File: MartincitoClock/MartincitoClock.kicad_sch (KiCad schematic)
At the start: 31 parts, among them J2 PJ-102AH, SW1 Omron_B3F_SPST, U1 ATmega328-PU, U2 L7805, Y1 Crystal

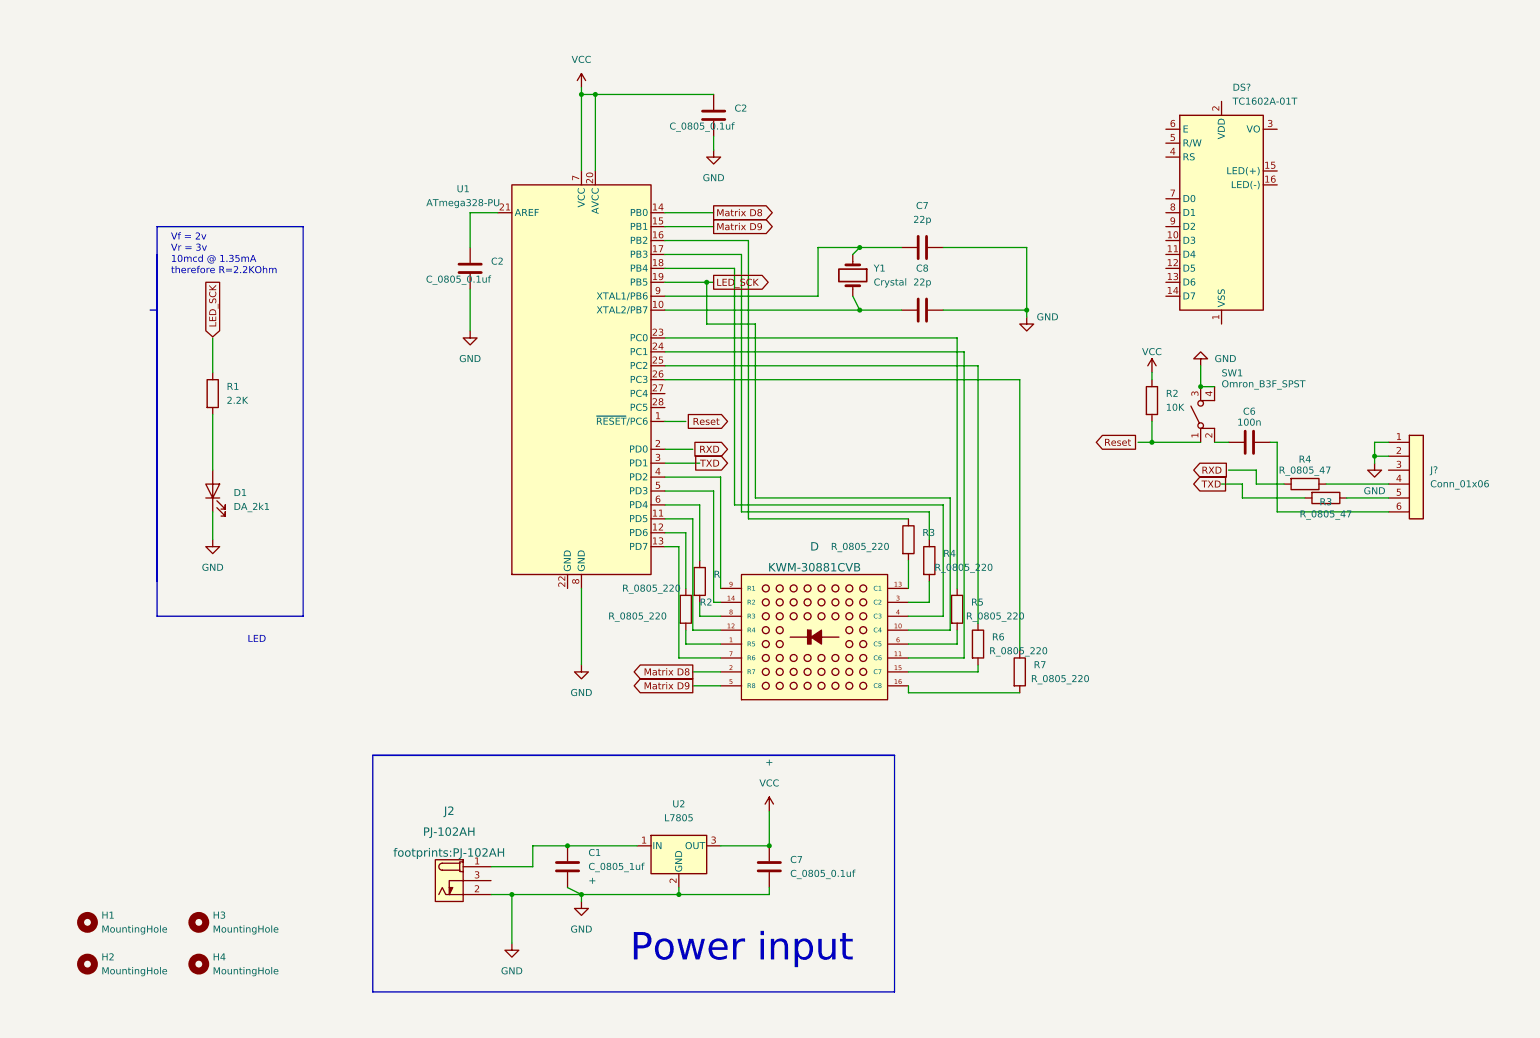
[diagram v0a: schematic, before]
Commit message: Week 5
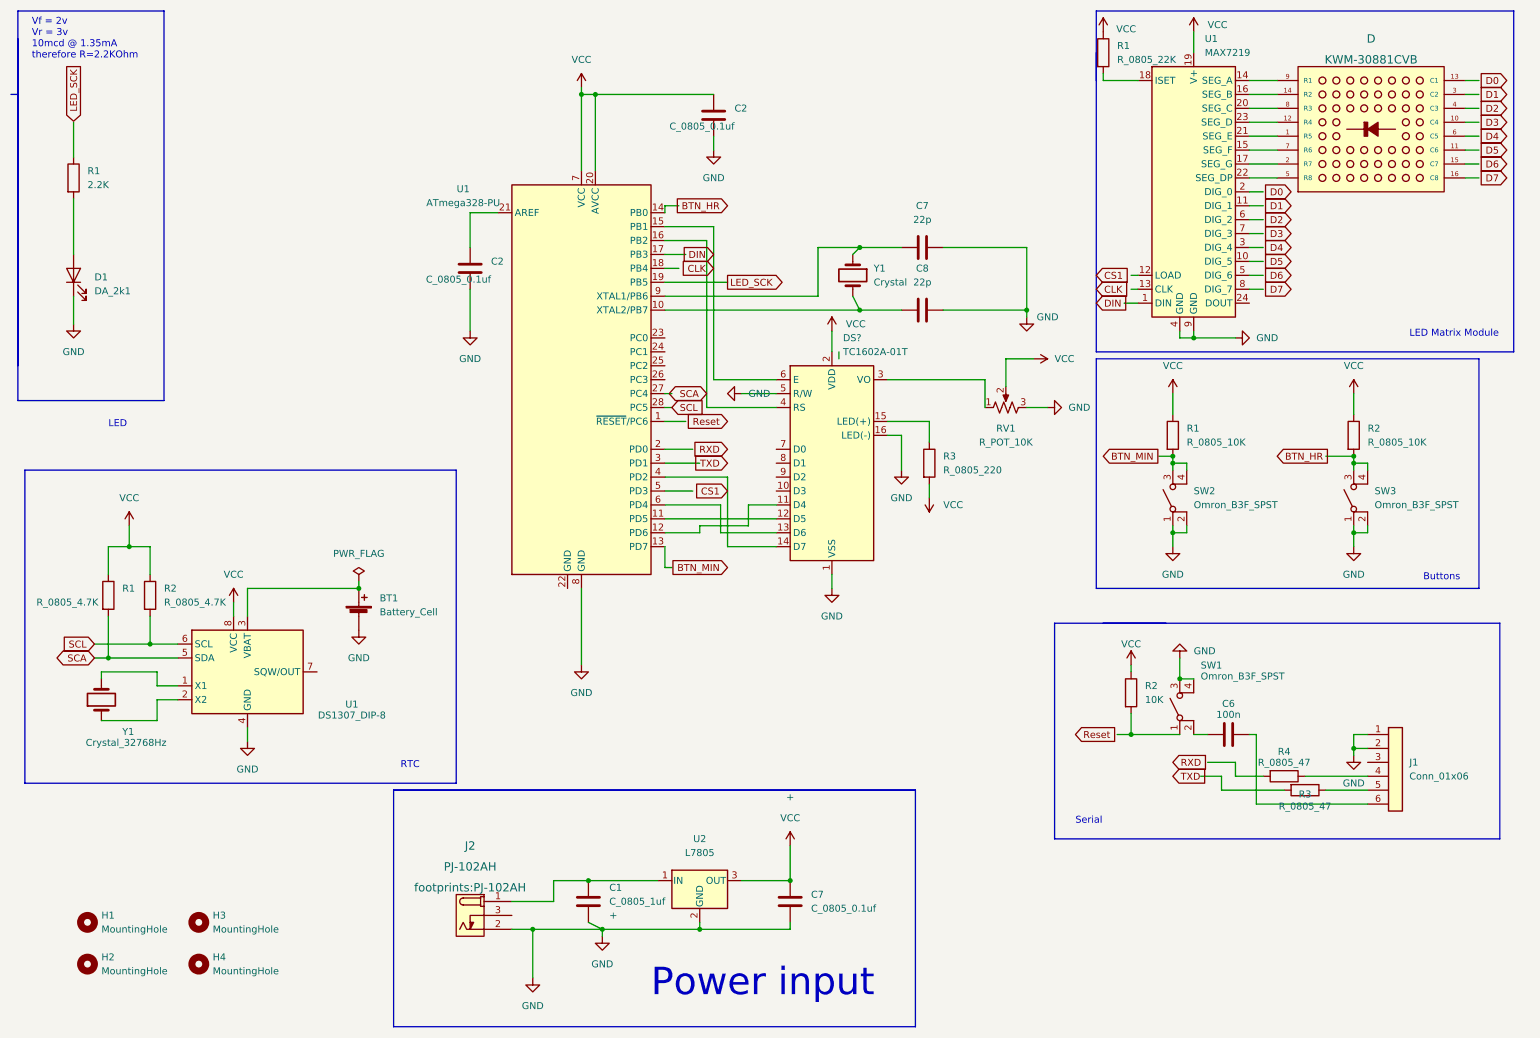
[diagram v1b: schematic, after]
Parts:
- removed DS?: TC1602A-01T, footprints:TC1602A-01T, symbol HPS:TC1602A-01T
- removed R, R2, R4, R5, R6, R7: R_0805_220, footprints:R_0805_2012Metric, symbol HPS:R_0805_100K
- added BT1: Battery_Cell, footprints:BatteryHolder_Keystone_106_1x20mm, symbol HPS:Battery_Cell
- added DS?: TC1602A-01T, footprints:TC1602A-01T, symbol HPS:TC1602A-01T
- added R1, R2: R_0805_4.7K, footprints:R_0805_2012Metric, symbol HPS:R_0805_4.7K
- added R1: R_0805_22K, footprints:R_0805_2012Metric, symbol HPS:R_0805_22K
- added R1, R2: R_0805_10K, footprints:R_0805_2012Metric, symbol HPS:R_0805_10K
- added RV1: R_POT_10K, footprints:Potentiometer_Bourns_3386P_Vertical, symbol HPS:R_POT_10K
- added SW2, SW3: Omron_B3F_SPST, footprints:SW_SPST_Omron_B3FS-100xP, symbol HPS:Omron_B3F_SPST
- added U1: DS1307_DIP-8, footprints:DIP-8_W7.62mm, symbol HPS:DS1307_DIP-8
- added U1: MAX7219, footprints:DIP-24_W7.62mm, symbol HPS:MAX7219
- added Y1: Crystal_32768Hz, footprints:Crystal_SMD_2Pin_3.2x1.5mm, symbol HPS:Crystal_32768Hz
- gave numbers to parts that had none: 1
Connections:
- net GND: now also BT1.2 (-), DS?.1 (VSS), DS?.16 (LED(-)), DS?.5 (R/W), RV1.3, SW2.1 (A), SW2.2 (A), SW3.1 (A), SW3.2 (A), U1.4 (GND), U1.4 (GND), U1.9 (GND)
- net LED_SCK: no longer D.10 (C4)
- net VCC: now also R3.2, DS?.2 (VDD), R1.1, R1.1, R1.1, R2.1, R2.1, RV1.2, U1.19 (V+), U1.8 (VCC)
- net at U1.11 (PD5): now also DS?.12 (D5); no longer D.12 (R4)
- net at U1.12 (PD6): now also DS?.11 (D4)
- net at U1.13 (PD7): no longer D.7 (R6)
- net at R3.1: now also DS?.15 (LED(+)); no longer U1.16 (PB2)
- net at U1.18 (PB4): no longer D.4 (C3)
- net at U1.24 (PC1): no longer D.11 (C6)
- net SCL: now reaches U1.28 (PC5)
- net SCL: now also R2.2, U1.6 (SCL)
- net at D.9 (R1): now also U1.14 (SEG_A); no longer U1.4 (PD2)
- net at U1.5 (PD3): no longer D.14 (R2)
- net at U1.6 (PD4): now also DS?.13 (D6)
- net at D.1 (R5): now also U1.21 (SEG_E)
- net at D.13 (C1): no longer R3.2
- net at D.8 (R3): now also U1.20 (SEG_C)
- net Matrix D8: no longer names the net of U1.14 (PB0)
- net Matrix D8: no longer D.2 (R7)
- net Matrix D9: no longer names the net of D.5 (R8)
- net Matrix D9: now also U1.22 (SEG_DP); no longer U1.15 (PB1)
- new net: R2.2, SW3.3 (B), SW3.4 (B)
- new net: DS?.3 (VO), RV1.1
- new net: R1.2, U1.18 (ISET)
- new net: D.12 (R4), U1.23 (SEG_D)
- new net: D.14 (R2), U1.16 (SEG_B)
- new net: D.2 (R7), U1.17 (SEG_G)
- new net: D.7 (R6), U1.15 (SEG_F)
- new net: U1.1 (X1), Y1.2
- new net: U1.2 (X2), Y1.1
- new net: BT1.1 (+), U1.3 (VBAT)
- new net: R1.2, SW2.3 (B), SW2.4 (B)
- new net CLK: DS?.6 (E), U1.15 (PB1)
- new net CS1: DS?.14 (D7), U1.4 (PD2)
- new net SCA: DS?.4 (RS), R1.2, U1.16 (PB2), U1.5 (SDA)
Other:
- note added: "Buttons"
- note added: "LED Matrix Module"
- note added: "RTC"
- note added: "Serial"
- moved on the sheet: C1, C6, C7, D, D1, J1, J2, R1, R2, R3, R4, SW1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
